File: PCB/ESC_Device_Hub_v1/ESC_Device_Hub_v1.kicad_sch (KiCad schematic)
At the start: 130 parts, among them J1 Conn_01x04, J10 Conn_01x06, J11 Conn_01x02, J12 Conn_01x02, J13 Conn_01x02, J14 Conn_01x02, J15 Conn_01x02, J16 Conn_01x02, J17 Conn_01x02, J18 Conn_01x02, J19 Conn_01x05, J2 Conn_01x04, J20 Conn_01x01, J21 Conn_01x01, J22 Conn_01x02, J3 Conn_01x04, J4 Conn_01x04, J5 Conn_01x04, J6 Conn_01x04, J7 Conn_01x06, J8 Conn_01x06, J9 Conn_01x06, SW1 SW_Push, SW2 SW_Push, SW4 SW_DIP_x02, U1 ISO1042BQDWVQ1, U10 LM66100DCK, U11 LM66100DCK, U18 USB_Type-C, U2 MCP2562FD-H/MF, U3 IS25LP064D-JLLE, U4 STM32H563RGVx, U6 TLP293, U7 NJM2884U1-33, U8 RFM-0505S, Y1 FC2012SN 32.768K-70NNA0KC0, Y2 XRCGB25M000FFS1AR0

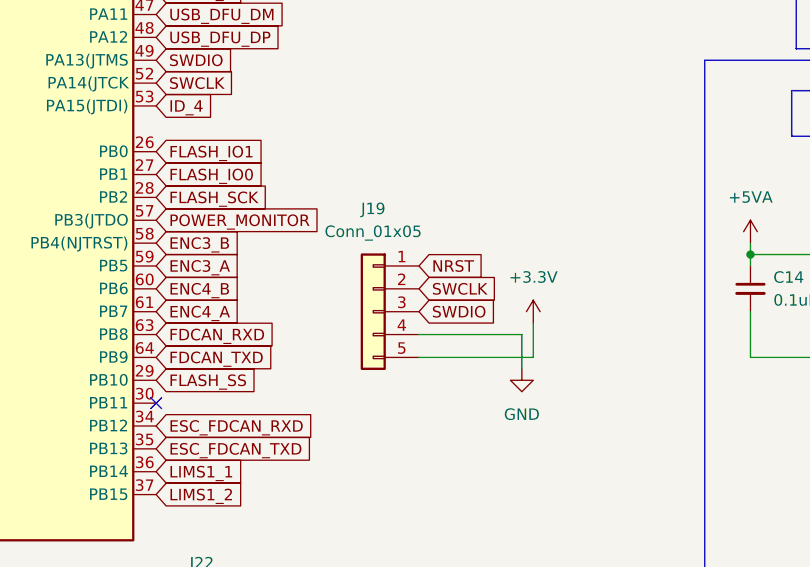
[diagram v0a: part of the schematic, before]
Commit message: 原因不明
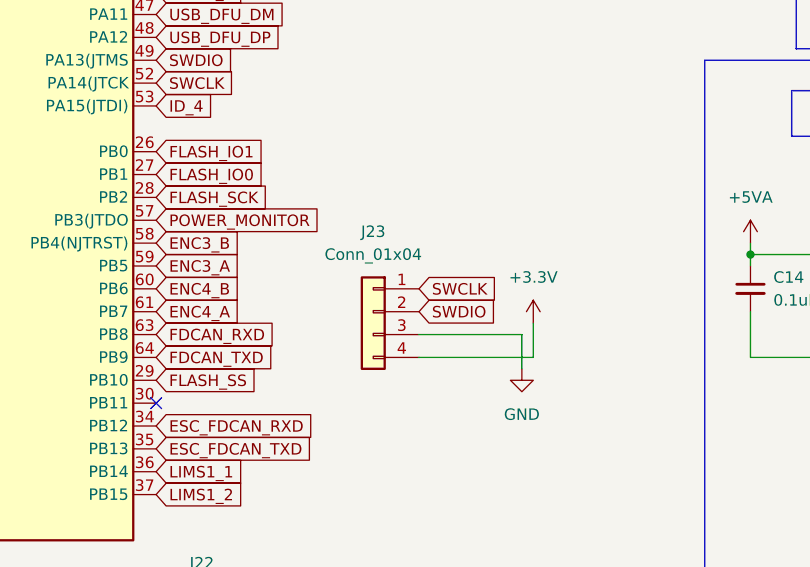
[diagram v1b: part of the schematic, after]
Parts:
- removed J19: Conn_01x05, Connector_PinSocket_2.54mm:PinSocket_1x05_P2.54mm_Vertical, symbol Connector_Generic:Conn_01x05
- added J23: Conn_01x04, Connector_PinSocket_2.54mm:PinSocket_1x04_P2.54mm_Vertical, symbol Connector_Generic:Conn_01x04
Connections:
- net +3.3V: now also J23.4 (Pin_4)
- net GND: now also J23.3 (Pin_3)
- net SWCLK: now also J23.1 (Pin_1)
- net SWDIO: now also J23.2 (Pin_2)
